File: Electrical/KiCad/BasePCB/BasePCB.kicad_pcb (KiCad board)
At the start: 2 copper layers, 54 x 58 mm, 17 parts, among them J1 Conn_01x02_Socket, J10 Conn_01x08, J2 Conn_01x02_Socket, J3 Conn_01x06_Socket, J4 Conn_01x06_Socket, J5 Conn_01x06, J6 Conn_01x03, J7 Conn_01x03, J8 Conn_01x04, J9 Conn_01x08, Q1 AO3400A, Q2 AO3400A

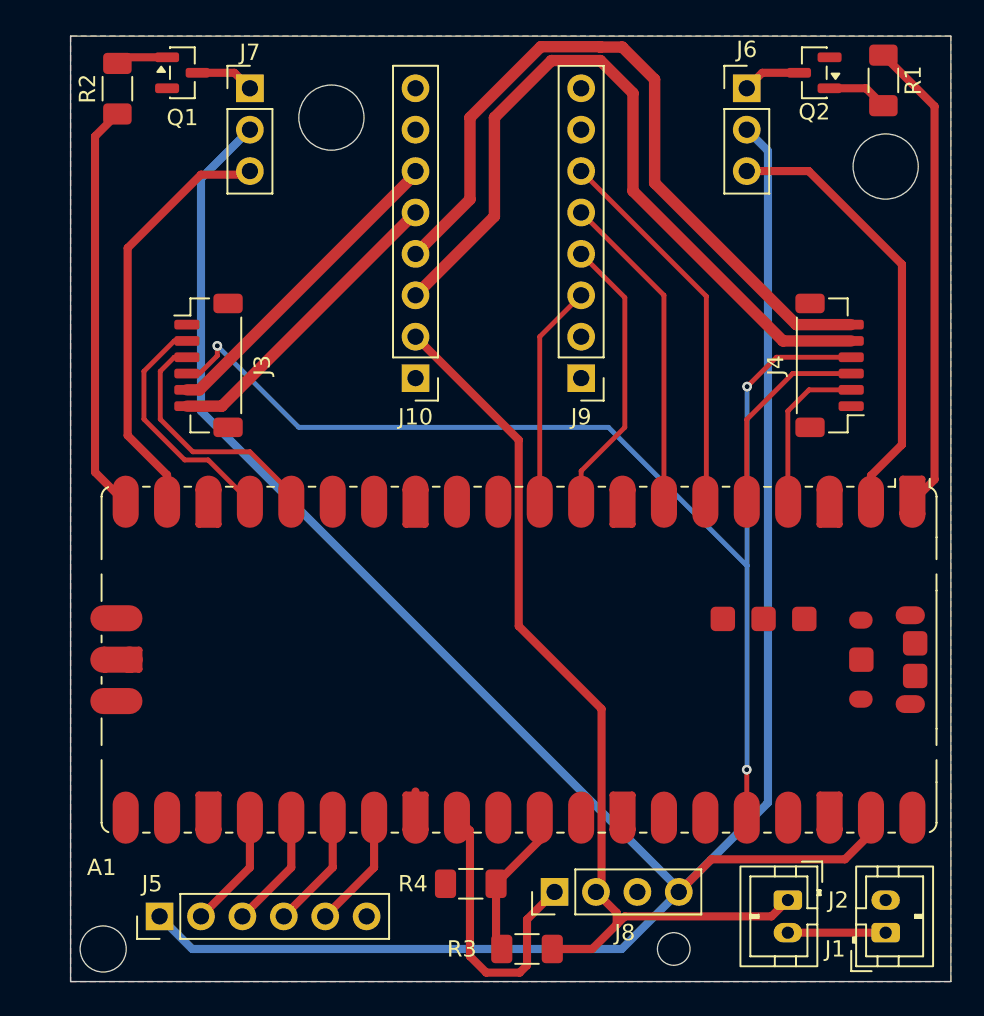
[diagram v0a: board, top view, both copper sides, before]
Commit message: Add the base PCB gerbers and JLCPCB production files
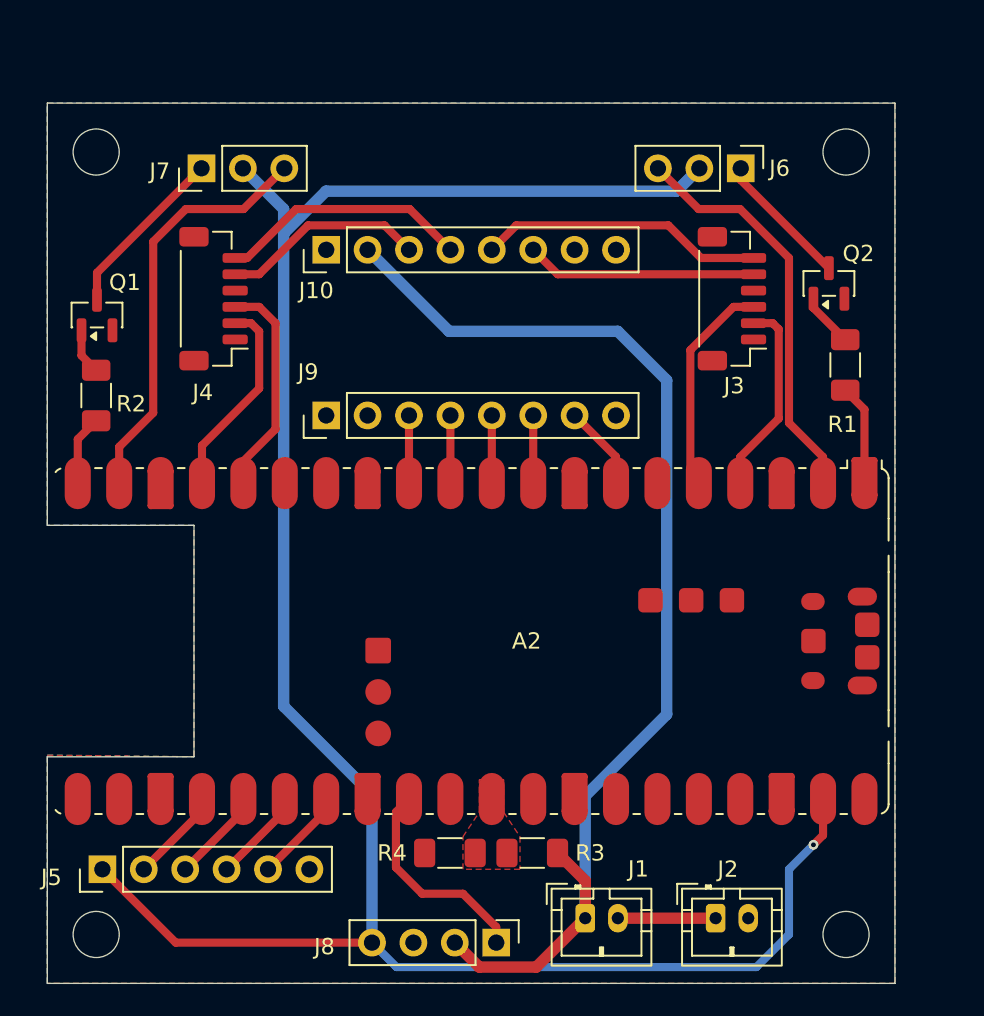
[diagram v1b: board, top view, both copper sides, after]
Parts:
- removed A1: RaspberryPi_Pico, Module:RaspberryPi_Pico_SMD
- added A2: RaspberryPi_Pico_W, Module:RaspberryPi_Pico_W_SMD, F.Cu at (140.6, 110.1)
- R3: value 570k -> 100k
- R4: value 330k -> 56k
- moved J4 38.0 mm to (124.8, 89.1)
- moved J3 32.4 mm to (156.6, 89.1), turned to 90 degrees
- moved R2 18.9 mm to (117.6, 95.0)
- moved R1 17.6 mm to (163.5, 93.2), turned to 90 degrees
- moved J9 15.8 mm to (131.7, 96.3), turned to 90 degrees
- moved Q1 15.8 mm to (117.6, 90.1), turned to 90 degrees
- moved Q2 13.0 mm to (162.5, 88.2), turned to 90 degrees
- moved J1 12.5 mm to (147.6, 127.1), turned to 0 degrees
- moved J2 10.5 mm to (155.6, 127.1), turned to 0 degrees
- moved J10 9.59 mm to (131.7, 86.1), turned to 90 degrees
- moved R3 5.90 mm to (144.3, 123.1)
- moved J7 5.74 mm to (124.0, 81.1), turned to 90 degrees
- moved J6 4.92 mm to (157.1, 81.1), turned to -90 degrees
- moved J8 4.74 mm to (142.1, 128.6), turned to -90 degrees
- moved J5 4.55 mm to (118.0, 124.1)
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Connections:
- J3 pad MP: (no net) -> GND
- J4 pad MP: (no net) -> GND
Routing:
- net +3.3V: track 74.6 -> 0.00 mm, vias 3 -> 0
- net /MB1: track 46.9 -> 12.5 mm
- net /MB2: track 45.7 -> 15.5 mm
- net +5V: track 158.1 -> 132.5 mm, vias 0 -> 1
- net /SA_PWR: track 29.4 -> 6.19 mm
- net /SB_PWR: track 25.3 -> 4.29 mm
- net /AIN1: track 23.5 -> 4.15 mm
- net /AIN2: track 19.8 -> 4.15 mm
- net +BATT: track 57.1 -> 71.3 mm
- net /BIN2: track 17.4 -> 4.15 mm
- net /BIN1: track 13.7 -> 4.15 mm
- net /Vchg: track 9.31 -> 0.00 mm
- net Net-(J7-Pin_1): track 3.60 -> 10.7 mm
- net /MA1: track 19.7 -> 14.1 mm
- net /nSLEEP: track 0.00 -> 5.20 mm
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- added copper zone on F.Cu, net /Vchg
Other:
- board size 54 x 58 mm -> 52 x 54 mm
